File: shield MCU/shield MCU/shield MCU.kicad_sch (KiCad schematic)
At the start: 16 parts, among them J1 IR_sensor, J2 IR_sensor, J3 IR_sensor, J4 IR_sensor, J5 IR_sensor

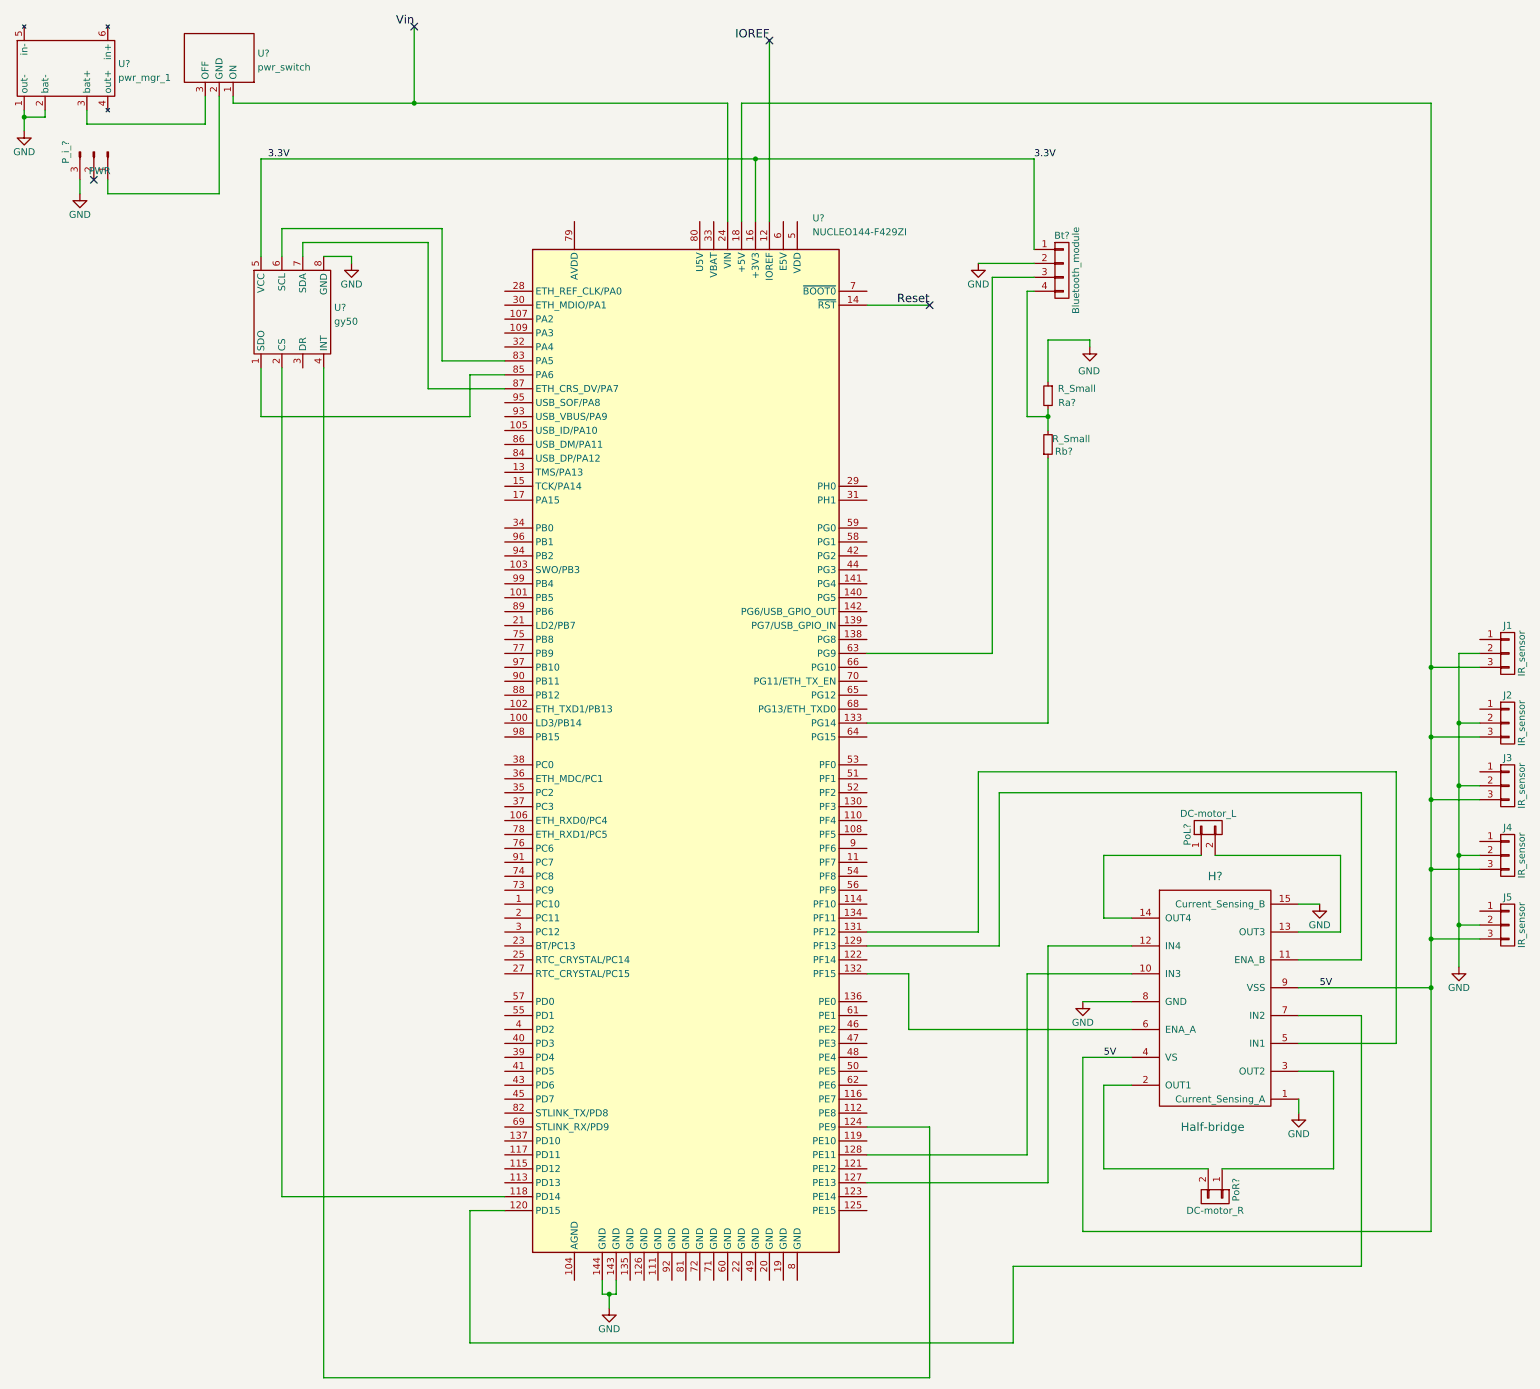
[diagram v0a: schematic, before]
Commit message: Valmis schema
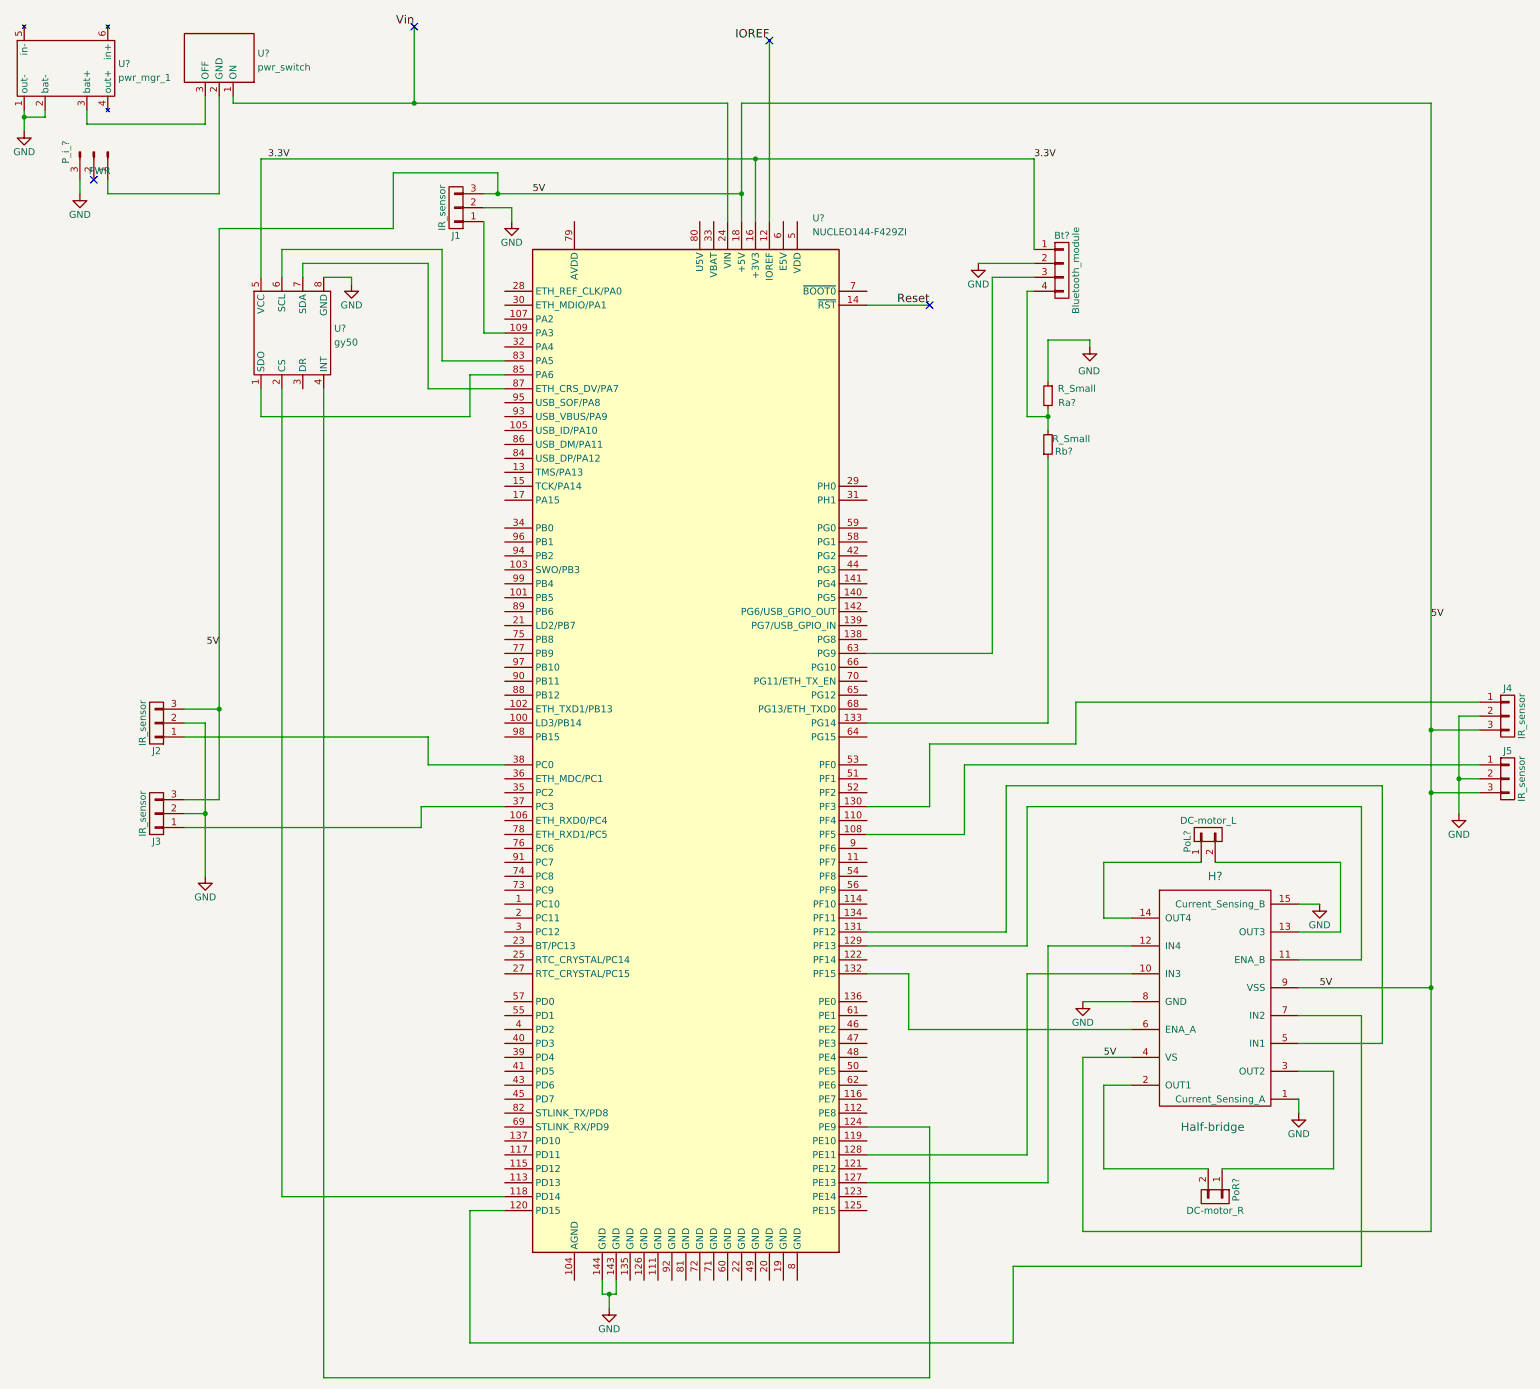
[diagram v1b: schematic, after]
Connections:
- net at J4.1 (P1): now also U?.130 (PF3)
- net at J3.1 (P1): now also U?.37 (PC3)
- net at J2.1 (P1): now also U?.38 (PC0)
- net at U?.108 (PF5): now also J5.1 (P1)
- net at U?.109 (PA3): now also J1.1 (P1)
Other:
- moved on the sheet: J1, J2, J3, J4, J5, PoL?, U?
